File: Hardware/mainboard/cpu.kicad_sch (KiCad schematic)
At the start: 52 parts, among them SW2 DNP, U100 IMXRT1050, Y100 24MHz, Y101 32.768K

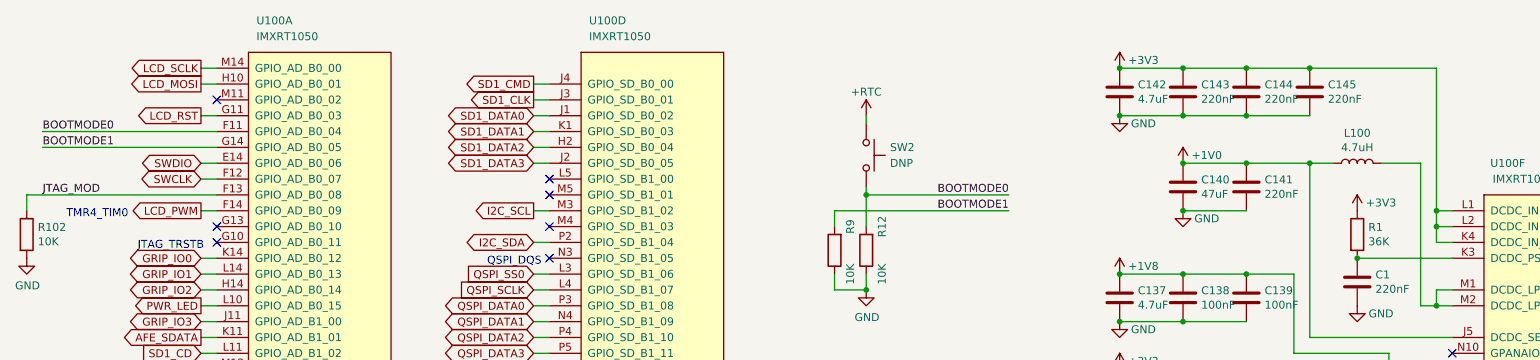
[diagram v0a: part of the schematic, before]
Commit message: Next set of PCB revisions WIP
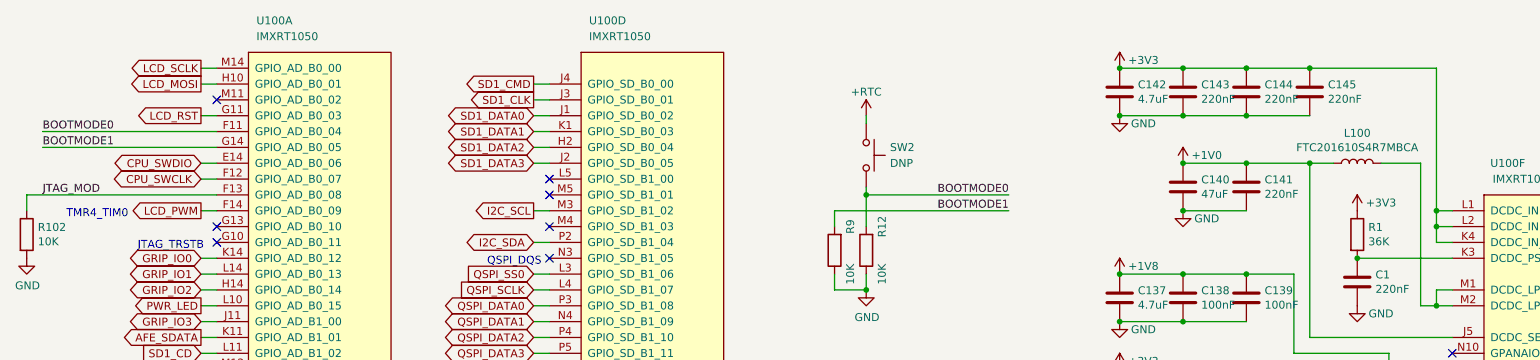
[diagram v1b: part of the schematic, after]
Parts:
- L100: value 4.7uH -> FTC201610S4R7MBCA; footprint footprints:L_1212 -> Inductor_SMD:L_Murata_DFE201610P
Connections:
- net SWCLK renamed CPU_SWCLK
- net SWDIO renamed CPU_SWDIO
